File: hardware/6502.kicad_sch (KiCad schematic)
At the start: 62 parts, among them J1 JMP, J10 JMP, J12 Control_bus, J13 EzRST, J14 Power, J15 Data_bus, J16 Address bus, J17 JMP, J18 JMP, J19 JMP, J2 PORTAB, J20 Interface, J3 CA, J4 CB, J5 W27c512?, J8 Barrel_Jack, J9 USB_B_Micro, SW1 SW_Push, U1 74HC14, U14 74HC04, U15 MIC5504-3.3YM5, U17 74HC00, U2 R6502, U3 R6522, U4 74HC273, U5 SST39SF010, U8 74HC32, U9 NRF24L01_Breakout

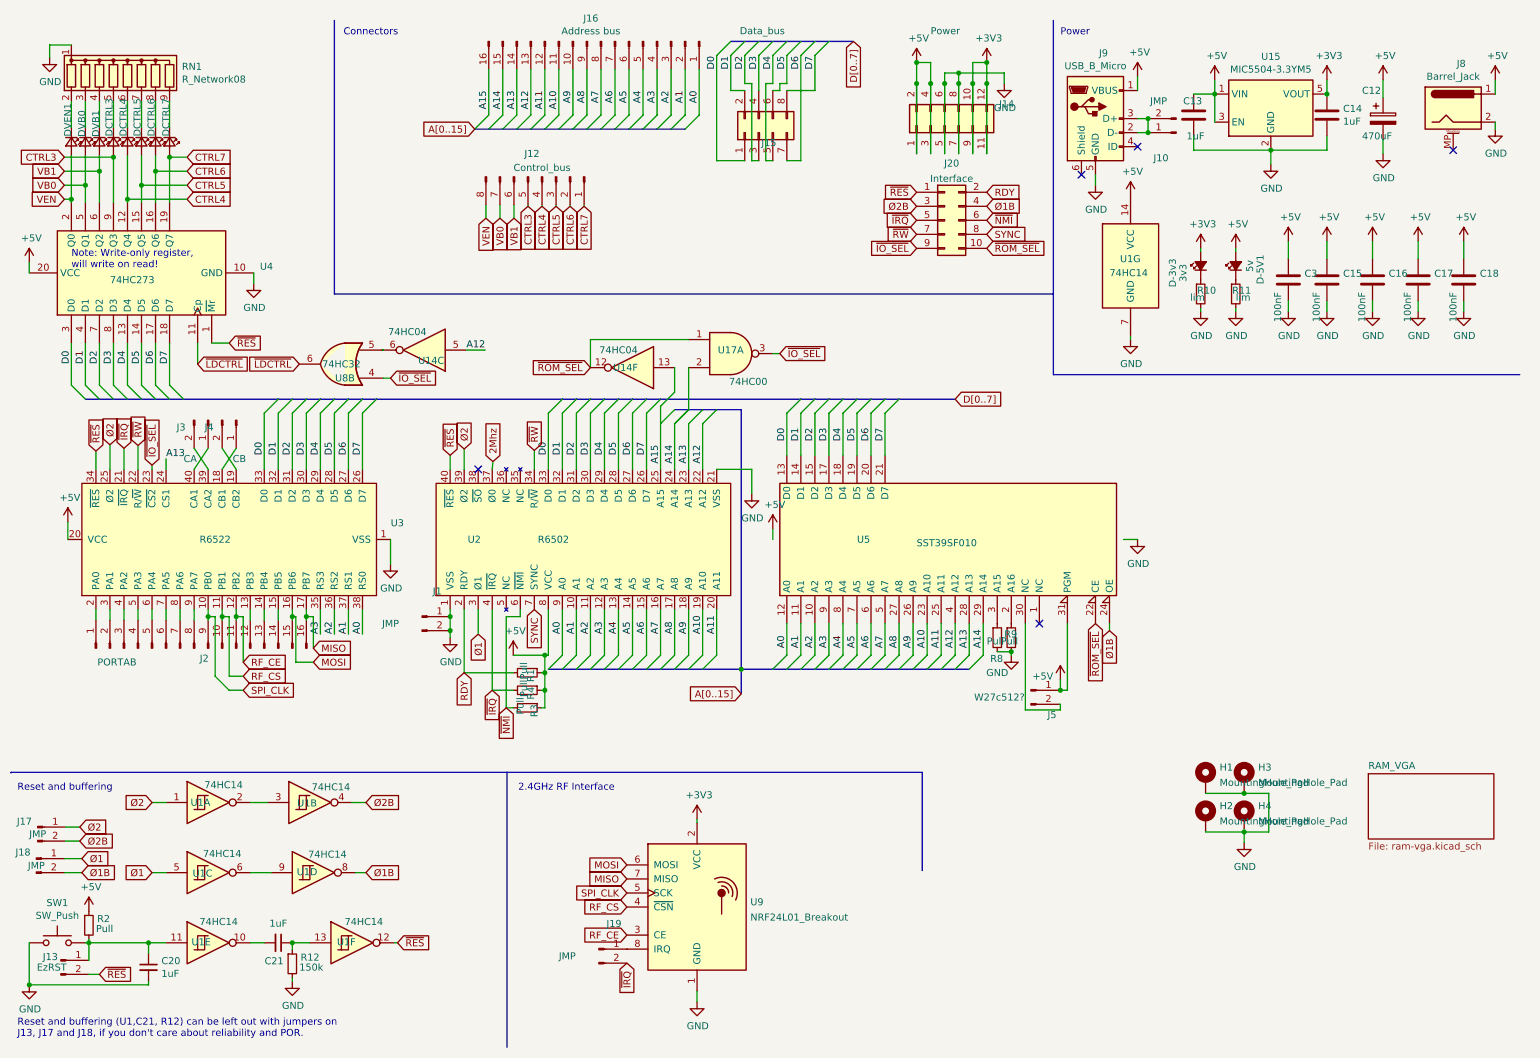
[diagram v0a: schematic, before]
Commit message: R1B2 gerbers, start+stop bits in modem driver
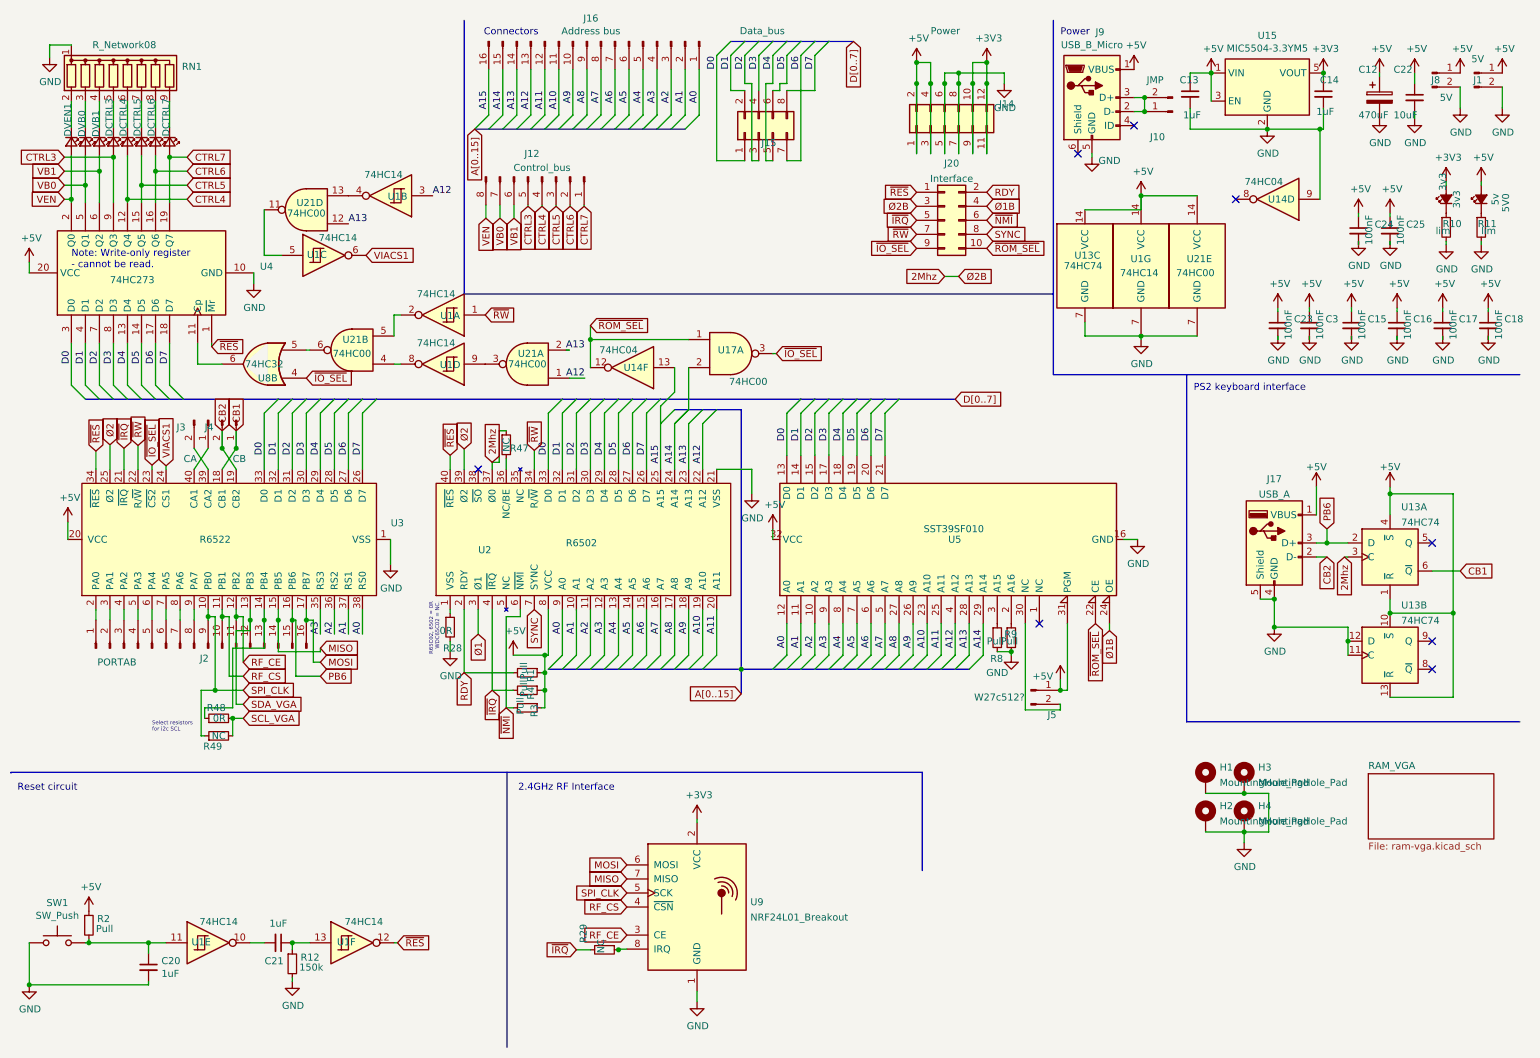
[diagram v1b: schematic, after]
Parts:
- removed J13: EzRST, Connector_PinHeader_2.54mm:PinHeader_1x02_P2.54mm_Vertical, symbol Connector:Conn_01x02_Male
- removed J17, J18, J19: JMP, Connector_PinHeader_2.54mm:PinHeader_1x02_P2.54mm_Vertical, symbol Connector:Conn_01x02_Male
- removed J8: Barrel_Jack, Connector_BarrelJack:BarrelJack_Horizontal, symbol Connector:Barrel_Jack_MountingPin
- removed unit 3 of U14
- added C22: 10uF, Capacitor_SMD:C_0805_2012Metric, symbol Device:C_Small
- added C23, C24, C25: 100nF, Capacitor_SMD:C_0603_1608Metric, symbol Device:C_Small
- added J17: USB_A, Connector_USB:USB_A_Molex_67643_Horizontal, symbol Connector:USB_A
- added J8: 5V, Connector_PinHeader_2.54mm:PinHeader_1x02_P2.54mm_Vertical, symbol Connector:Conn_01x02_Male
- added R28: 0R, Resistor_SMD:R_0402_1005Metric_Pad0.72x0.64mm_HandSolder, symbol Device:R_Small
- added R29, R47: NC, Resistor_SMD:R_0402_1005Metric_Pad0.72x0.64mm_HandSolder, symbol Device:R_Small
- added R48: 0R, Resistor_SMD:R_0805_2012Metric, symbol Device:R_Small
- added R49: NC, Resistor_SMD:R_0805_2012Metric, symbol Device:R_Small
- added U13: 74HC74, Package_DIP:DIP-14_W7.62mm, symbol 74xx:74HC74
- added unit 4 of U14
- added U21: 74HC00, Package_DIP:DIP-14_W7.62mm, symbol 74xx:74HC00
- C13, C14, C15, C16, C17, C18, C3: symbol Device:C -> Device:C_Small
- J1: value JMP -> 5V
- renumbered D-3v3 to 3v3, D-5V1 to 5V0
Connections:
- net +5V: now also J1.1 (Pin_1), C22.1, C23.1, C24.1, C25.1, J17.1 (VBUS), J8.1 (Pin_1), U13.1 (~{R}), U13.10 (~{S}), U13.13 (~{R}), U13.14 (VCC), U13.4 (~{S}), U21.14 (VCC)
- net 2Mhz: now also J20.3 (Pin_3), R47.1, U13.3 (C)
- net A12: now also U1.3, U21.1
- net A13: now also U21.12, U21.2; no longer U3.24 (CS1)
- net GND: now also C22.2, C23.2, C24.2, C25.2, J17.4 (GND), J17.5 (Shield), J8.2 (Pin_2), R28.2, U13.11 (C), U13.12 (D), U13.7 (GND), U14.9, U21.7 (GND); no longer J1.1 (Pin_1), U2.1 (VSS)
- net MISO: now also J2.14 (Pin_14), U3.15 (PB5); no longer J2.16 (Pin_16), U3.17 (PB7)
- net MOSI: now also J2.16 (Pin_16), U3.17 (PB7); no longer J2.15 (Pin_15), U3.16 (PB6)
- net SPI_CLK: now also R49.1
- net ~{IRQ}: now also R29.2
- net ~{RW}: now also U1.1
- net Ø1: no longer U1.5
- net Ø1B: no longer U1.8
- net Ø2: no longer U1.1
- net at U2.36 (NC/BE): now also R47.2
- net SDA_VGA: now reaches J2.12 (Pin_12), U3.13 (PB3)
- net at J2.13 (Pin_13), U3.14 (PB4): now also R48.1
- net CB1: now reaches J4.1 (Pin_1), U3.18 (CB1)
- net CB1: now also U13.6 (~{Q})
- net CB2: now reaches J4.2 (Pin_2), U3.19 (CB2)
- net CB2: now also J17.2 (D-)
- net at U1.2: now also U21.5; no longer U1.3
- net at U1.9: now also U21.3; no longer U1.6
- net at U9.8 (IRQ): now also R29.1
- net at U8.5: now also U21.6
- net ~{LDCTRL}: no longer names the net of U4.11 (Cp), U8.6
- net Ø2B: no longer names the net of U1.4
- net Ø2B: now also U21.13; no longer J20.3 (Pin_3)
- new net: R28.1, U2.1 (VSS)
- new net: U1.8, U21.4
- new net: U1.5, U21.11
- new net PB6: J17.3 (D+), J2.15 (Pin_15), U13.2 (D), U3.16 (PB6)
- new net SCL_VGA: R48.2, R49.2
- new net VIACS1: U1.6, U3.24 (CS1)
- no-connect marks 5 -> 8
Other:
- note added: "Note: Write-only register - cannot be read."
- note added: "PS2 keyboard interface"
- note added: "R65C02, 6502 = 0R WDC65C02 = NC."
- note added: "Reset circuit"
- note added: "Select resistors for i2c SCL"
- note removed: "Note: Write-only register, will write on read!"
- note removed: "Reset and buffering"
- note removed: "Reset and buffering (U1,C21, R12) can be left out with jumpers on J13, J17 and J18, if you don't care about reliability and POR."
- moved on the sheet: 3v3, 5V0, C12, C13, C14, C15, C16, C17, C18, C3, J10, J9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
